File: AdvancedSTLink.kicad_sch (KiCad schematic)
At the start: 63 parts, among them J1 Conn_01x03, J3 Conn_01x06, J4 USB_C_Receptacle_USB2.0, J5 Conn_01x05, Q1 S8050, SW1 SW_SPDT, SW2 SW_Push, U1 STM32F205RETx, U2 XC6206P332MR, U3 USBLC6-2P6, U5 USBLC6-2P6, U6 USBLC6-2P6, U7 SY8032E, Y1 X322512MSB4SI

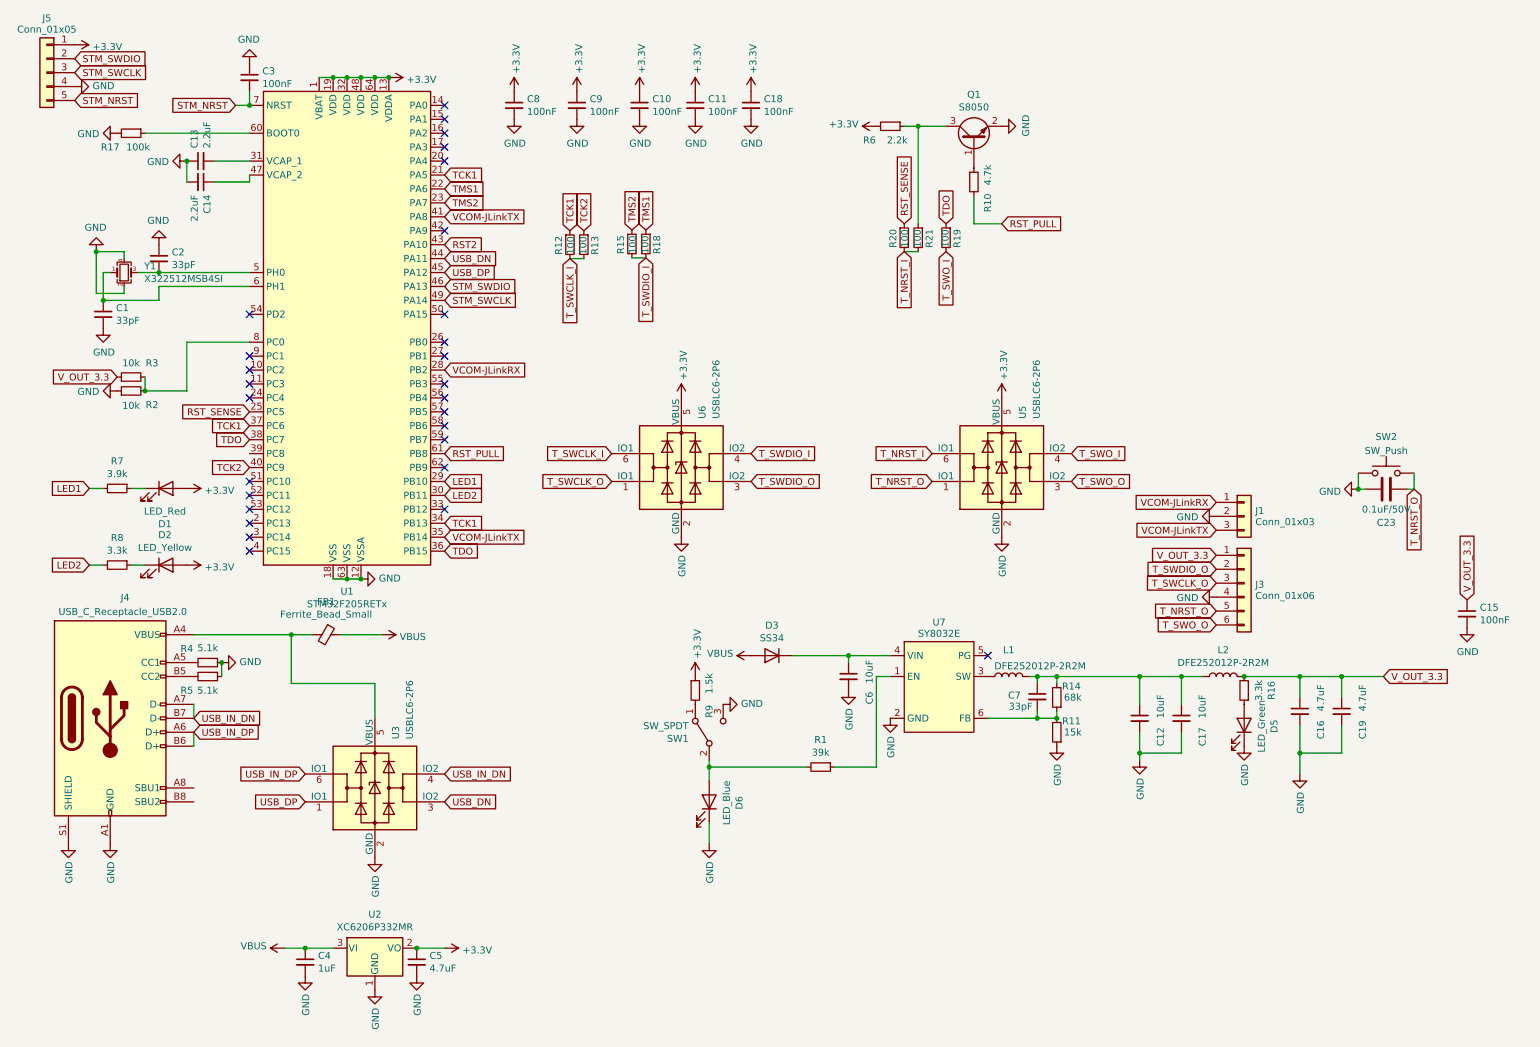
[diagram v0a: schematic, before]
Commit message: 增加一个hub
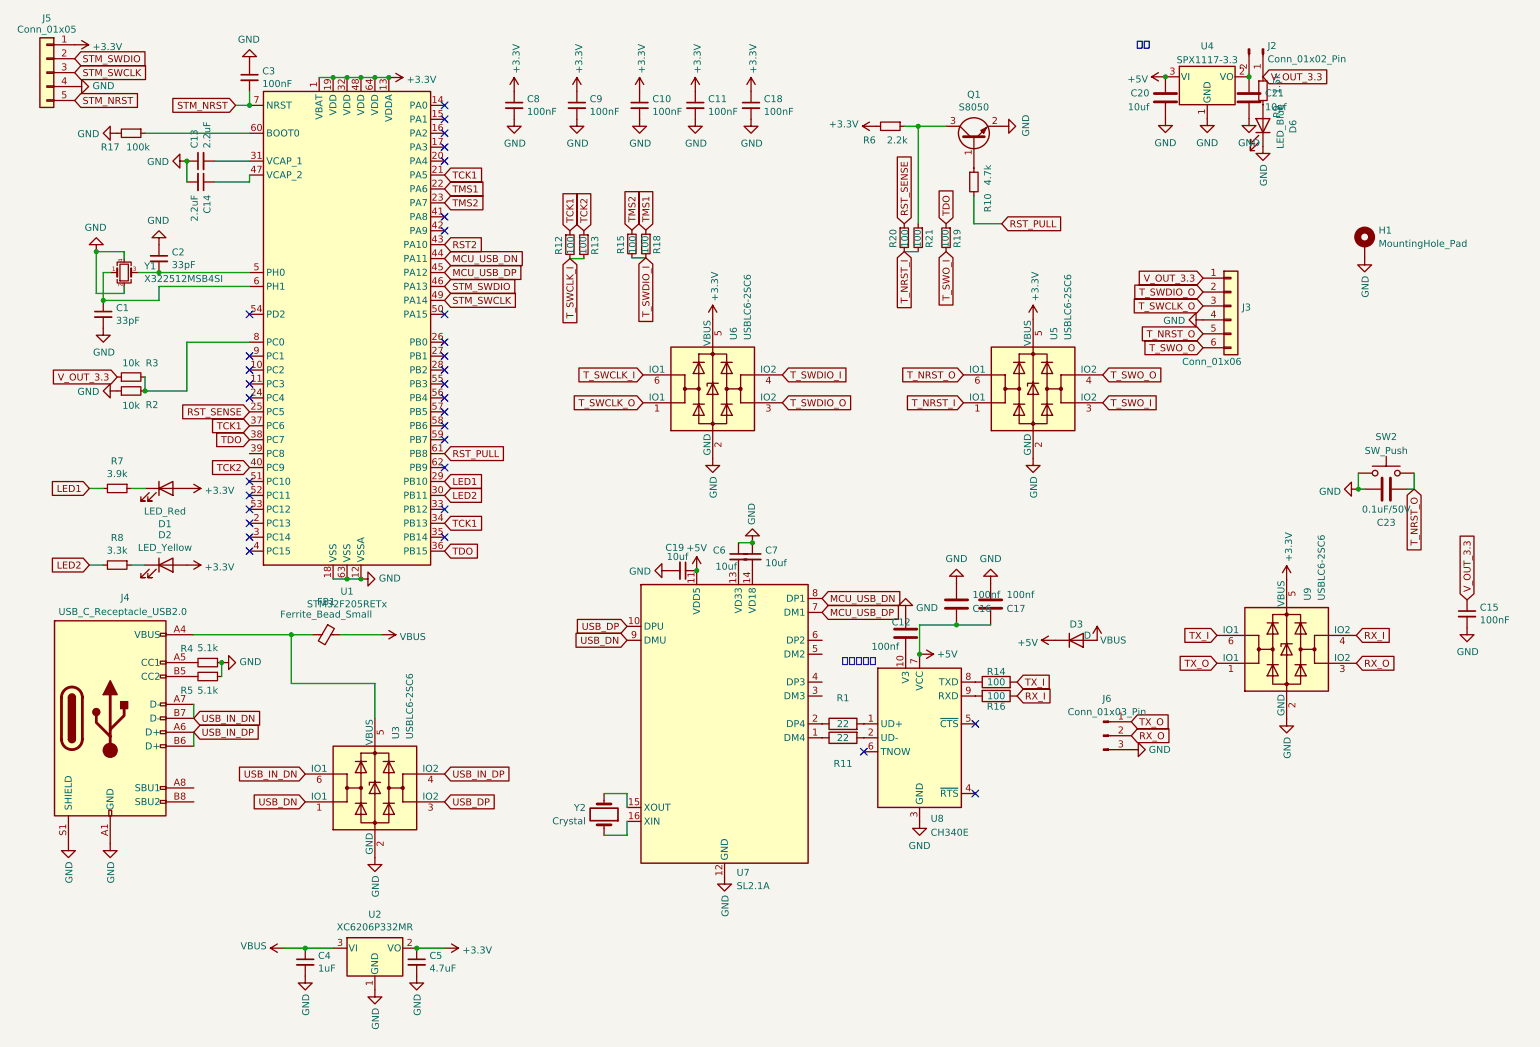
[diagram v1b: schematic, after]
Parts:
- removed C12, C17: 10uF, Capacitor_SMD:C_0805_2012Metric, symbol Device:C_Small
- removed C16: 4.7uF, Capacitor_SMD:C_0603_1608Metric, symbol Device:C_Small
- removed D5: LED_Green, LED_SMD:LED_0603_1608Metric_Pad1.05x0.95mm_HandSolder, symbol Device:LED
- removed J1: Conn_01x03, Connector_PinHeader_2.54mm:PinHeader_1x03_P2.54mm_Vertical, symbol Connector_Generic:Conn_01x03
- removed L1, L2: DFE252012P-2R2M, lc:DFE252012P, symbol Device:L
- removed R1: 39k, Resistor_SMD:R_0402_1005Metric, symbol Device:R_Small
- removed R11: 15k, Resistor_SMD:R_0603_1608Metric, symbol Device:R_Small
- removed R14: 68k, Resistor_SMD:R_0603_1608Metric, symbol Device:R_Small
- removed R16: 3.3k, Resistor_SMD:R_0402_1005Metric, symbol Device:R_Small
- removed SW1: SW_SPDT, Button_Switch_SMD:SW_SPDT_CK-JS102011SAQN, symbol Switch:SW_SPDT
- removed U7: SY8032E, lc:SOT-23-6, symbol t123yh_lib2:SY8032E
- added C12, C16, C17: 100nf, Capacitor_SMD:C_0402_1005Metric, symbol Device:C
- added C20, C21: 10uf, Capacitor_SMD:C_0805_2012Metric, symbol Device:C
- added H1: MountingHole_Pad, MountingHole:MountingHole_2.2mm_M2_Pad_Via, symbol Mechanical:MountingHole_Pad
- added J2: Conn_01x02_Pin, Connector_PinHeader_2.54mm:PinHeader_1x02_P2.54mm_Vertical, symbol Connector:Conn_01x02_Pin
- added J6: Conn_01x03_Pin, Connector_PinHeader_2.54mm:PinHeader_1x03_P2.54mm_Vertical, symbol Connector:Conn_01x03_Pin
- added R1, R11: 22, Resistor_SMD:R_0402_1005Metric, symbol Device:R
- added R14, R16: 100, Resistor_SMD:R_0402_1005Metric, symbol Device:R
- added U4: SPX1117-3.3, Package_TO_SOT_SMD:SOT-223-3_TabPin2, symbol Regulator_Linear:AZ1117-3.3
- added U7: SL2.1A, Package_SO:SOP-16_4.4x10.4mm_P1.27mm, symbol Interface_USB:FE1.1s
- added U8: CH340E, Package_SO:MSOP-10_3x3mm_P0.5mm, symbol Interface_USB:CH340E
- added U9: USBLC6-2SC6, lc:SOT-23-6, symbol AdvancedSTLink-rescue:USBLC6-2SC6-Power_Protection
- added Y2: Crystal, KisonNew:C16369, symbol Device:Crystal
- C19: value 4.7uF -> 10uf; footprint Capacitor_SMD:C_0603_1608Metric -> Capacitor_SMD:C_0805_2012Metric
- C6: value 10uF -> 10uf
- C7: value 33pF -> 10uf; footprint Capacitor_SMD:C_0402_1005Metric -> Capacitor_SMD:C_0805_2012Metric
- D3: value SS34 -> D; footprint lc:SMA(DO-214AC)_S1 -> Diode_SMD:D_SOD-323; LCSC C8678 -> C191023
- U3, U5, U6: value USBLC6-2P6 -> USBLC6-2SC6; footprint lc:SOT-666 -> lc:SOT-23-6
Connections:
- net +3V3: now also U9.5 (VBUS); no longer R9.1
- net GND: now also C6.1, C7.1, C12.1, C16.2, C17.2, C20.2, C21.2, H1.1, J6.3 (Pin_3), U4.1 (GND), U7.12 (GND), U8.3 (GND), U9.2 (GND); no longer C6.2
- net T_NRST_I: now also U5.1 (IO1); no longer U5.6 (IO1)
- net T_NRST_O: now also U5.6 (IO1); no longer U5.1 (IO1)
- net T_SWO_I: now also U5.3 (IO2); no longer U5.4 (IO2)
- net T_SWO_O: now also U5.4 (IO2); no longer U5.3 (IO2)
- net USB_DN: now also U3.1 (IO1), U7.9 (DMU); no longer U1.44 (PA11), U3.3 (IO2)
- net USB_DP: now also U3.3 (IO2), U7.10 (DPU); no longer U1.45 (PA12), U3.1 (IO1)
- net USB_IN_DN: now also U3.6 (IO1); no longer U3.4 (IO2)
- net USB_IN_DP: now also U3.4 (IO2); no longer U3.6 (IO1)
- net V_OUT_3.3: now also R9.1, J2.1 (Pin_1); no longer C19.1
- net at R9.2: now also D6.2 (A)
- net +5V: now reaches D3.1 (K)
- net +5V: now also C19.1, C16.1, C17.1, C20.1, U4.3 (VI), U7.11 (VDD5), U8.7 (VCC); no longer C6.1
- net at C7.2: now also U7.14 (VD18)
- net VCOM-JLinkRX: no longer names the net of U1.28 (PB2)
- net VCOM-JLinkTX: no longer names the net of U1.35 (PB14)
- net VCOM-JLinkTX: no longer U1.41 (PA8)
- new net: R14.1, U8.8 (TXD)
- new net: C21.1, J2.2 (Pin_2), U4.2 (VO)
- new net: C12.2, U8.10 (V3)
- new net: R11.1, U7.1 (DM4)
- new net: R11.2, U8.2 (UD-)
- new net: C6.2, U7.13 (VD33)
- new net: R1.2, U8.1 (UD+)
- new net: R16.2, U8.9 (RXD)
- new net: U7.16 (XIN), Y2.1
- new net: U7.15 (XOUT), Y2.2
- new net: R1.1, U7.2 (DP4)
- new net MCU_USB_DN: U1.44 (PA11), U7.8 (DP1)
- new net MCU_USB_DP: U1.45 (PA12), U7.7 (DM1)
- new net RX_I: R16.1, U9.4 (IO2)
- new net RX_O: J6.2 (Pin_2), U9.3 (IO2)
- new net TX_I: R14.2, U9.6 (IO1)
- new net TX_O: J6.1 (Pin_1), U9.1 (IO1)
- no-connect marks 28 -> 33
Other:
- note added: "上位机串口"
- note added: "电源"
- moved on the sheet: D6, J3, R9, U5, U6

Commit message: 更新原理图
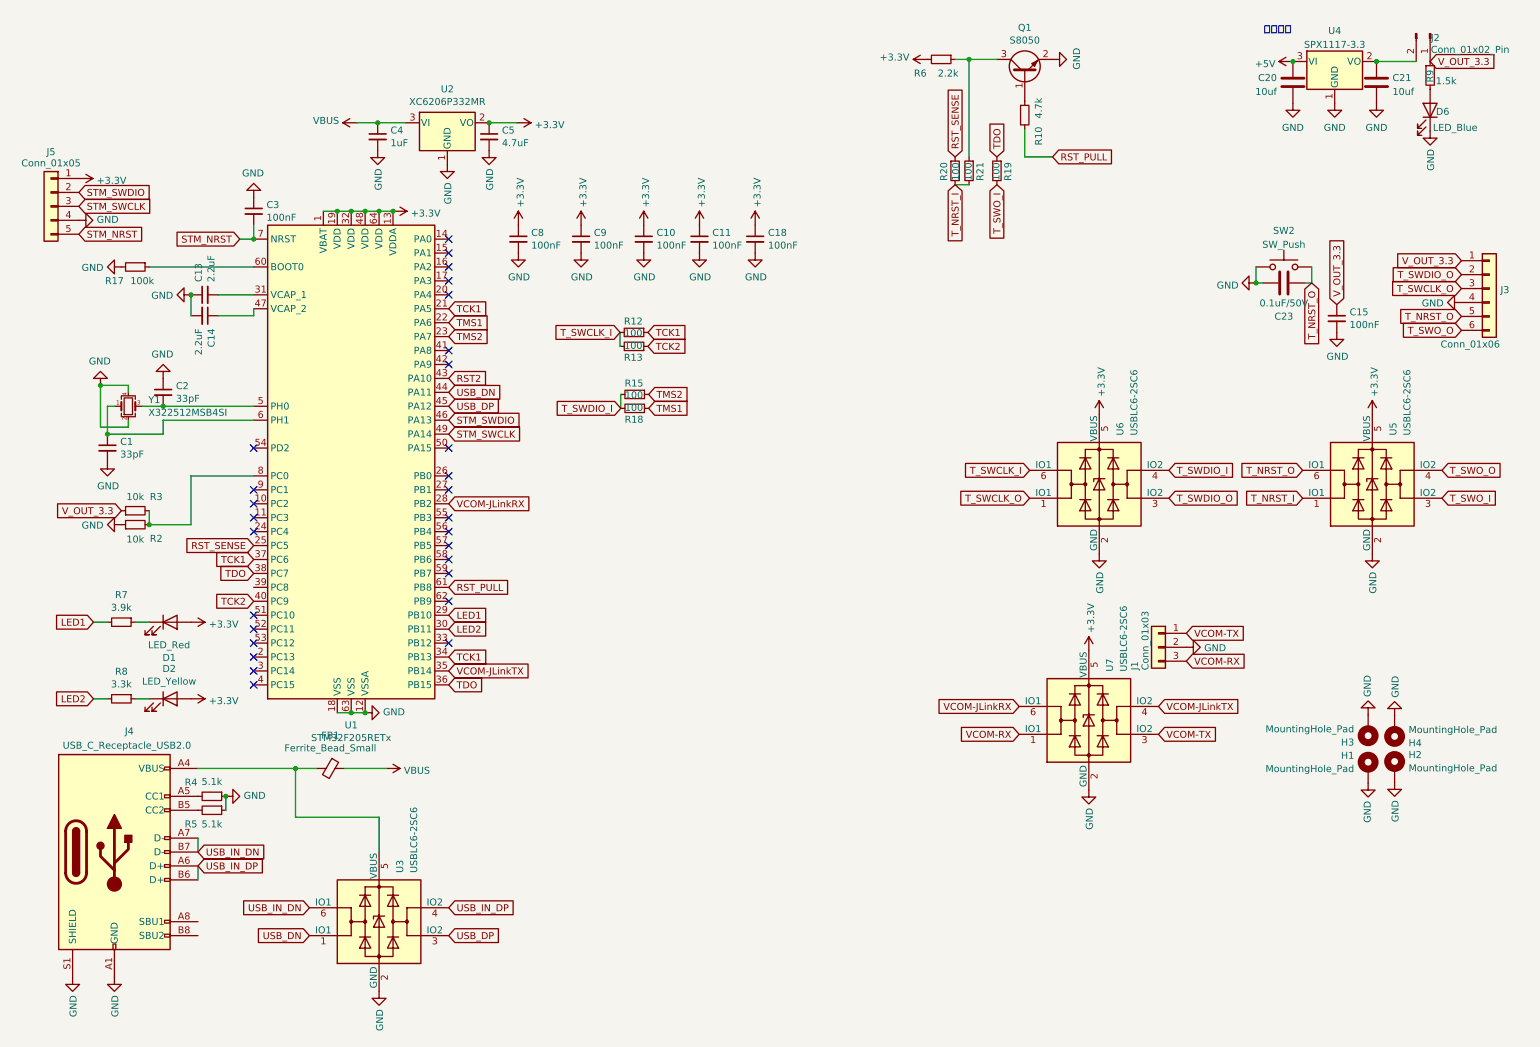
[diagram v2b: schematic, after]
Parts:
- removed C12, C16, C17: 100nf, Capacitor_SMD:C_0402_1005Metric, symbol Device:C
- removed C19, C6, C7: 10uf, Capacitor_SMD:C_0805_2012Metric, symbol Device:C_Small
- removed D3: D, Diode_SMD:D_SOD-323, symbol Device:D
- removed J6: Conn_01x03_Pin, Connector_PinHeader_2.54mm:PinHeader_1x03_P2.54mm_Vertical, symbol Connector:Conn_01x03_Pin
- removed R1, R11: 22, Resistor_SMD:R_0402_1005Metric, symbol Device:R
- removed R14, R16: 100, Resistor_SMD:R_0402_1005Metric, symbol Device:R
- removed U7: SL2.1A, Package_SO:SOP-16_4.4x10.4mm_P1.27mm, symbol Interface_USB:FE1.1s
- removed U8: CH340E, Package_SO:MSOP-10_3x3mm_P0.5mm, symbol Interface_USB:CH340E
- removed U9: USBLC6-2SC6, lc:SOT-23-6, symbol AdvancedSTLink-rescue:USBLC6-2SC6-Power_Protection
- removed Y2: Crystal, KisonNew:C16369, symbol Device:Crystal
- added H2, H3, H4: MountingHole_Pad, MountingHole:MountingHole_2.2mm_M2_Pad_Via, symbol Mechanical:MountingHole_Pad
- added J1: Conn_01x03, Connector_PinHeader_2.54mm:PinHeader_1x03_P2.54mm_Vertical, symbol Connector_Generic:Conn_01x03
- added U7: USBLC6-2SC6, lc:SOT-23-6, symbol AdvancedSTLink-rescue:USBLC6-2SC6-Power_Protection
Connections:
- net MCU_USB_DN is gone; now on net USB_DN: U1.44 (PA11)
- net MCU_USB_DP is gone; now on net USB_DP: U1.45 (PA12)
- net +3V3: now also U7.5 (VBUS)
- net GND: now also H2.1, H3.1, H4.1, J1.2 (Pin_2), U7.2 (GND)
- net VCOM-JLinkRX: now reaches U1.28 (PB2)
- net VCOM-JLinkRX: now also U7.6 (IO1)
- net VCOM-JLinkTX: now reaches U1.35 (PB14)
- net VCOM-JLinkTX: now also U7.4 (IO2)
- new net VCOM-RX: J1.3 (Pin_3), U7.1 (IO1)
- new net VCOM-TX: J1.1 (Pin_1), U7.3 (IO2)
- no-connect marks 33 -> 28
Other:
- note added: "对外电源"
- note removed: "上位机串口"
- note removed: "电源"
- moved on the sheet: C1, C10, C11, C13, C14, C15, C18, C2, C20, C21, C23, C3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
